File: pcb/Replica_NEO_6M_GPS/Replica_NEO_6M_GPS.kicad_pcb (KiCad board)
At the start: 2 copper layers, 46 x 36 mm, 24 parts, among them J1 CONUFL001-SMD-T, J2 Conn_01x04, U1 TPS79133DBVR, U2 NEO-6M-GPS, U3 24AA32A-I_MS

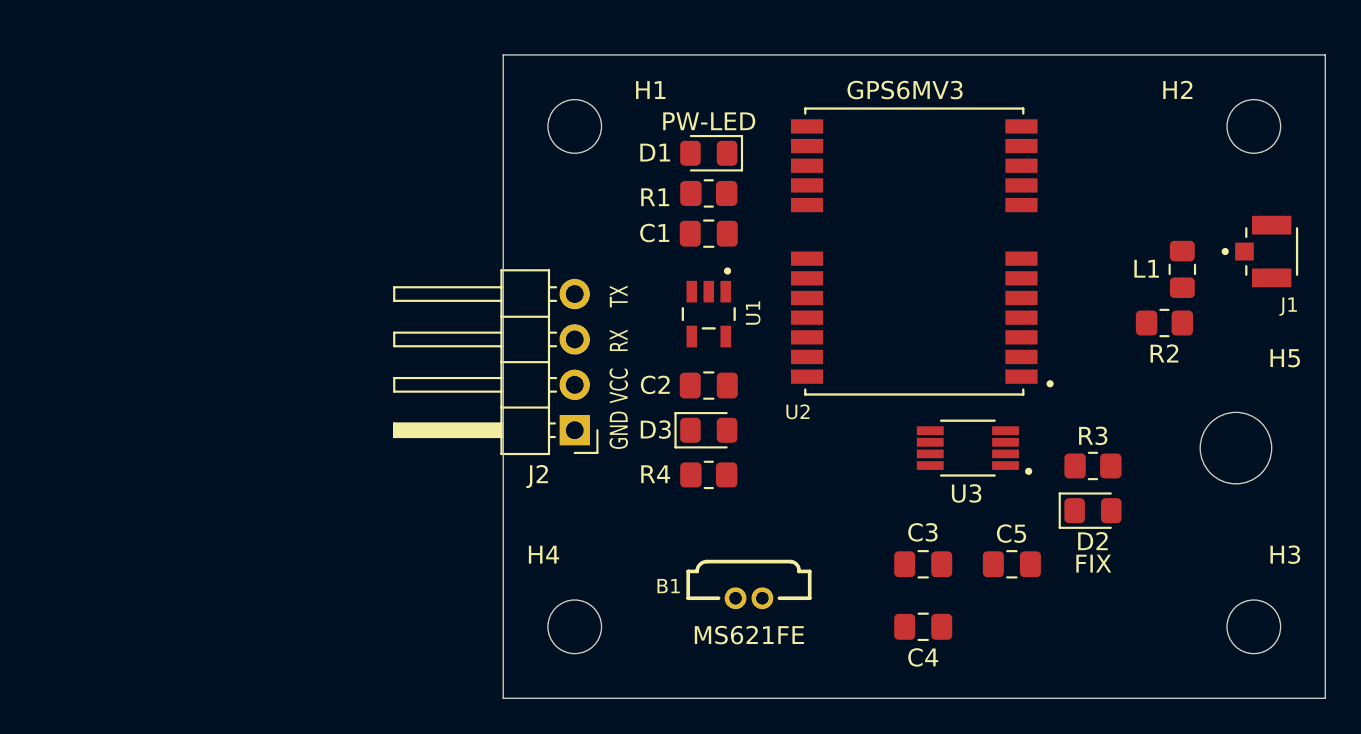
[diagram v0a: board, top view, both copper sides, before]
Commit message: Se hicieron correcciones
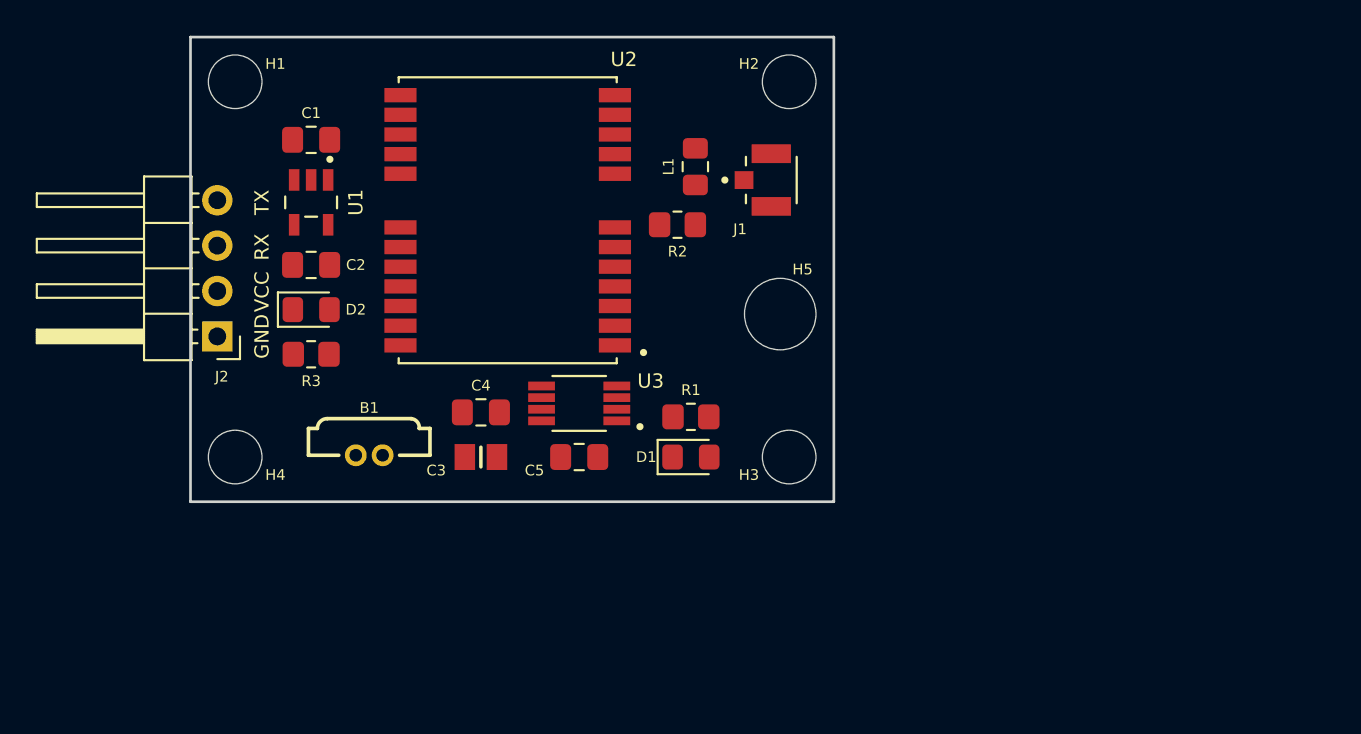
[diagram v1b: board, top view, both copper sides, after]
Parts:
- removed D3: 1N5817, Diode_SMD:D_0805_2012Metric_Pad1.15x1.40mm_HandSolder
- removed R4: 1K, Resistor_SMD:R_0805_2012Metric_Pad1.20x1.40mm_HandSolder
- B1: footprint MS621FE:MS621FE -> foot:MS621FE
- C4: footprint Capacitor_SMD:C_0805_2012Metric_Pad1.18x1.45mm_HandSolder -> foot:CAPC2012X140N
- D1: value LED -> FIX
- D2: value FIX -> 1N5817; footprint LED_SMD:LED_0805_2012Metric_Pad1.15x1.40mm_HandSolder -> Diode_SMD:D_0805_2012Metric_Pad1.15x1.40mm_HandSolder
- J1: footprint CONUFL001-SMD-T:LINX_CONUFL001-SMD-T -> foot:LINX_CONUFL001-SMD-T
- U1: footprint TPS79133DBVR:SOT95P280X145-5N -> foot:SOT95P280X145-5N
- U2: footprint NEO-6M-GPS d:XCVR_NEO-6M-GPS -> foot:XCVR_NEO-6M-GPS
- U3: footprint 24AA32A-I_MS:SOP65P490X110-8N -> foot:SOP65P490X110-8N
- moved D2 45.2 mm to (120.8, 100.2)
- moved R3 44.2 mm to (120.8, 102.8)
- moved J1 28.3 mm to (146.5, 93.0)
- moved L1 27.9 mm to (142.2, 92.2), turned to 90 degrees
- moved R2 27.8 mm to (141.2, 95.5)
- moved H3 27.7 mm to (147.5, 108.5)
- moved H5 26.6 mm to (147.0, 100.5)
- moved C4 26.5 mm to (130.2, 108.5), turned to 0 degrees
- moved C3 26.2 mm to (130.2, 106.0)
- moved H2 26.1 mm to (147.5, 87.5)
- moved C5 24.9 mm to (135.8, 108.5)
- moved C2 23.3 mm to (120.8, 97.8), turned to 0 degrees
- moved U1 23.1 mm to (120.8, 94.2)
- moved C1 22.9 mm to (120.8, 90.8), turned to 180 degrees
- moved U2 22.8 mm to (131.8, 95.2)
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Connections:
- net /Modulo GPS/RXD1 renamed /RXD1
- net /Modulo GPS/SCL2 renamed /SCL2
- net /Modulo GPS/SDA2 renamed /SDA2
- B1 pad -: Earth -> GND
- C1 pad 1: /Regulador de voltaje lineal de potencia/+5V -> VCC
- C1 pad 2: Earth -> GND
- C2 pad 2: Earth -> GND
- C3 pad 1: /Modulo GPS/3.3V -> +3V3
- C3 pad 2: Earth -> GND
- C4 pad 1: /Modulo GPS/3.3V -> GND
- C4 pad 2: Earth -> +3V3
- C5 pad 1: /Modulo GPS/3.3V -> +3V3
- C5 pad 2: Earth -> GND
- D1 pad 1: Earth -> GND
- D2 pad 1: Earth -> Net-(D2-Pad1)
- D2 pad 2: Net-(D2-Pad2) -> +3V3
- J1 pad 2: Earth -> GND
- J1 pad 3: Earth -> GND
- J2 pad 1: Earth -> VCC
- J2 pad 2: /Regulador de voltaje lineal de potencia/+5V -> /TXD1
- J2 pad 4: /Modulo GPS/TXD1 -> GND
- R1 pad 1: /Modulo GPS/3.3V -> Net-(R1-Pad1)
- R3 pad 1: Net-(R3-Pad1) -> Net-(D2-Pad1)
- R3 pad 2: Net-(D2-Pad2) -> Net-(B1-Pad+)
- U1 pad 1: /Regulador de voltaje lineal de potencia/+5V -> VCC
- U1 pad 2: Earth -> GND
- U1 pad 3: Earth -> GND
- U1 pad 5: /Modulo GPS/3.3V -> +3V3
- U2 pad 10: Earth -> GND
- U2 pad 12: Earth -> GND
- U2 pad 13: Earth -> GND
- U2 pad 20: /Modulo GPS/TXD1 -> /TXD1
- U2 pad 23: /Modulo GPS/3.3V -> +3V3
- U2 pad 24: Earth -> GND
- U2 pad 3: Net-(R3-Pad1) -> Net-(R1-Pad1)
- U2 pad 7: Earth -> GND
- U3 pad 1: Earth -> GND
- U3 pad 2: Earth -> GND
- U3 pad 3: Earth -> GND
- U3 pad 4: Earth -> GND
- U3 pad 7: Earth -> GND
- U3 pad 8: /Modulo GPS/3.3V -> +3V3
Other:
- board size 46 x 36 mm -> 36 x 26 mm
- board text added: "Comentarios: - No encuentro el footprint apropiado para la bateria, los que encuentro son mas grandes y no entran en el pcb (ademas de que no se corresponden con la pila que debe ir alli) Bordes y margenes: - Borde de PCB (1 mm) - Margen del PCB (1 mm) Cuadriculas de trabajo: - 0.250 mm para montaje. - 1 mm para dibujo de bordes y margenes"
- board text added: "Replica uBLOX NEO-6M GPS Module DCI - 3CEIoT UBA Christian Canaan UBA - Argentina"
- board text removed: "Comentarios: - Se incrementaron las dimensiones del PCB respecto al patron dado que se usan footprints mas grandes Bordes y margenes: - Borde de PCB (1 mm) - Margen del PCB (1 mm) Cuadriculas de trabajo: - 0.250 mm para montaje. - 1 mm para dibujo de bordes y margenes"
- board text removed: "FIX"
- board text removed: "GPS6MV3"
- board text removed: "MS621FE"
- board text removed: "PW-LED"
- board text removed: "Replica ublox GPS NEO 6M V3 Christian Canaan"
